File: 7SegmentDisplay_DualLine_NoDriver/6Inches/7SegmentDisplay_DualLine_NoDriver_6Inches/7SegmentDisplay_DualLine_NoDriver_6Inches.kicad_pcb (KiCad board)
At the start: 2 copper layers, 93.4 x 158.7 mm, 128 parts

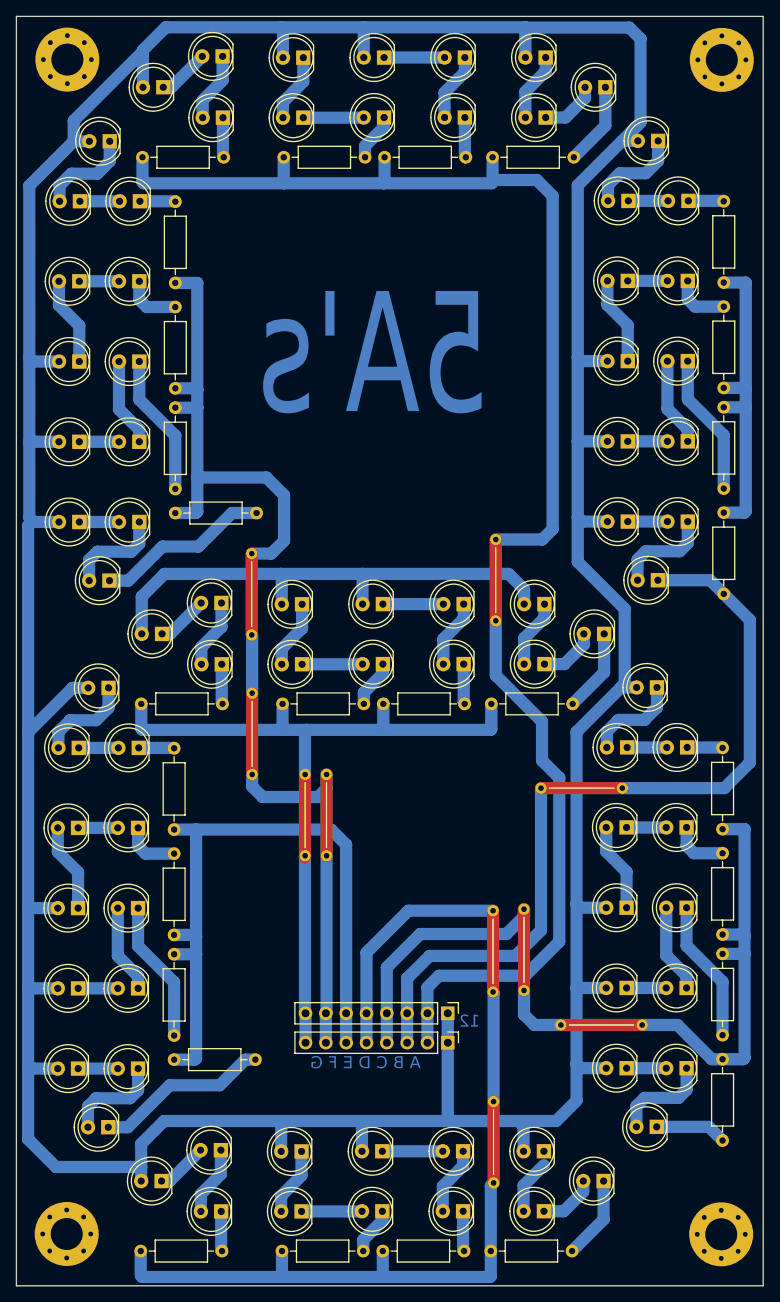
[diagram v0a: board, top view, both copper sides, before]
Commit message: ADDED: pdf files of the PCBs
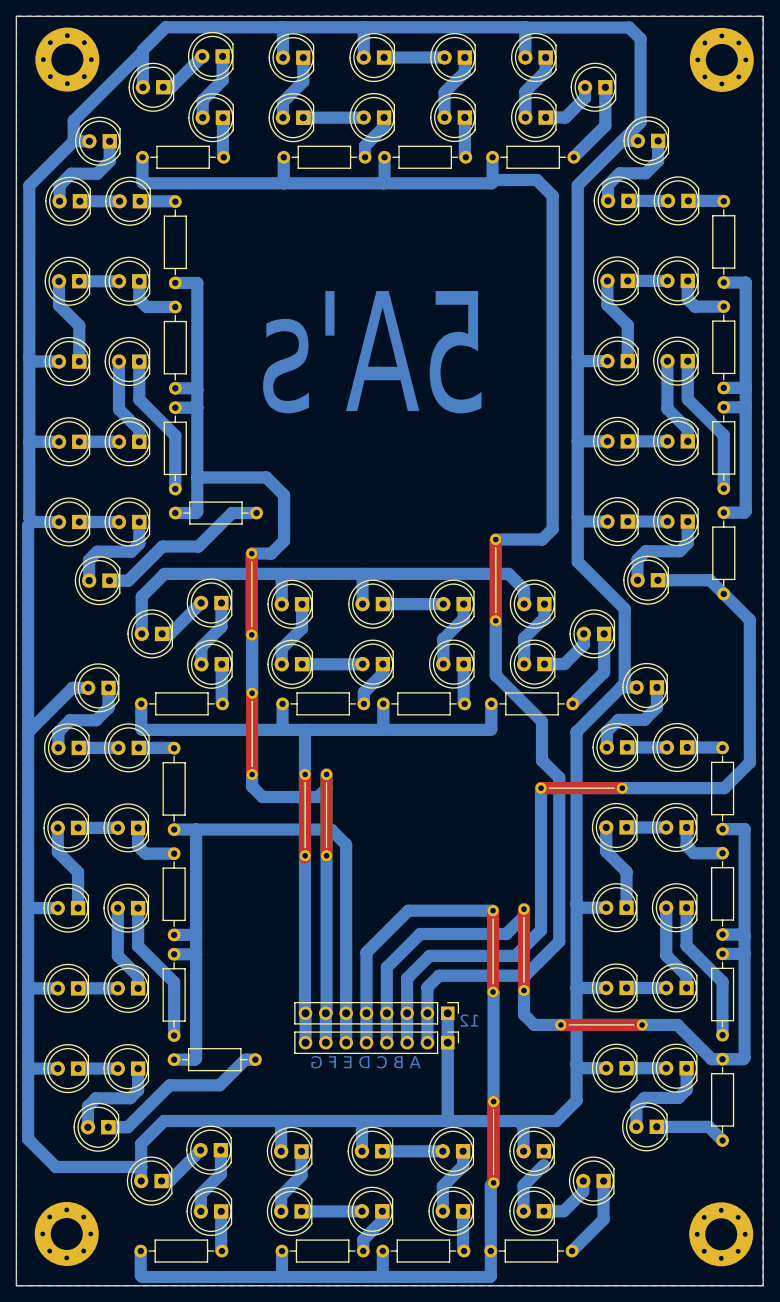
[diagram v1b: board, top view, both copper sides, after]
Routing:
- added copper zone on B.Cu, net (none)
